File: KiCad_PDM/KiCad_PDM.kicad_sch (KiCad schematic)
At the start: 67 parts, among them J1 Conn_02x16_Top_Bottom, J2 6437288-1, J3 T66145145-1500, U1 74HC27D, U2 74HC27D, U3 74HC27D, U4 74HC27D, U5 KF33BDT-TR

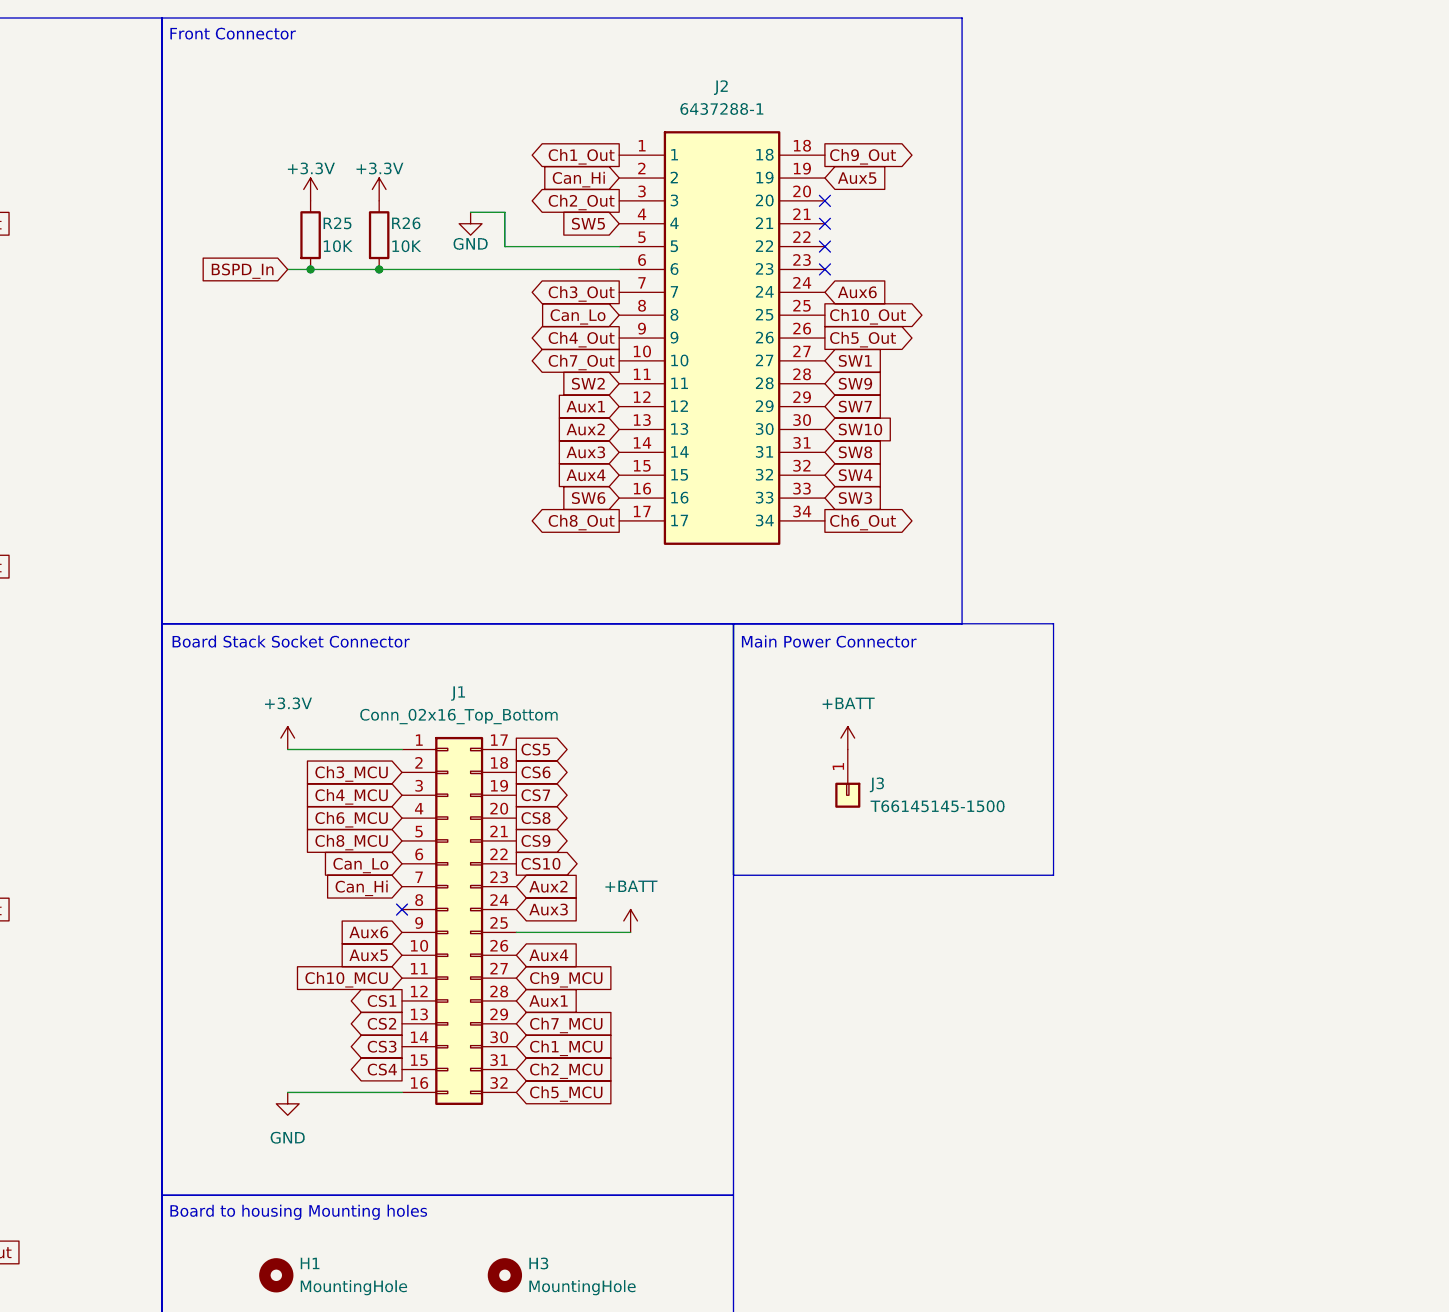
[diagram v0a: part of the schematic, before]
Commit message: MK1
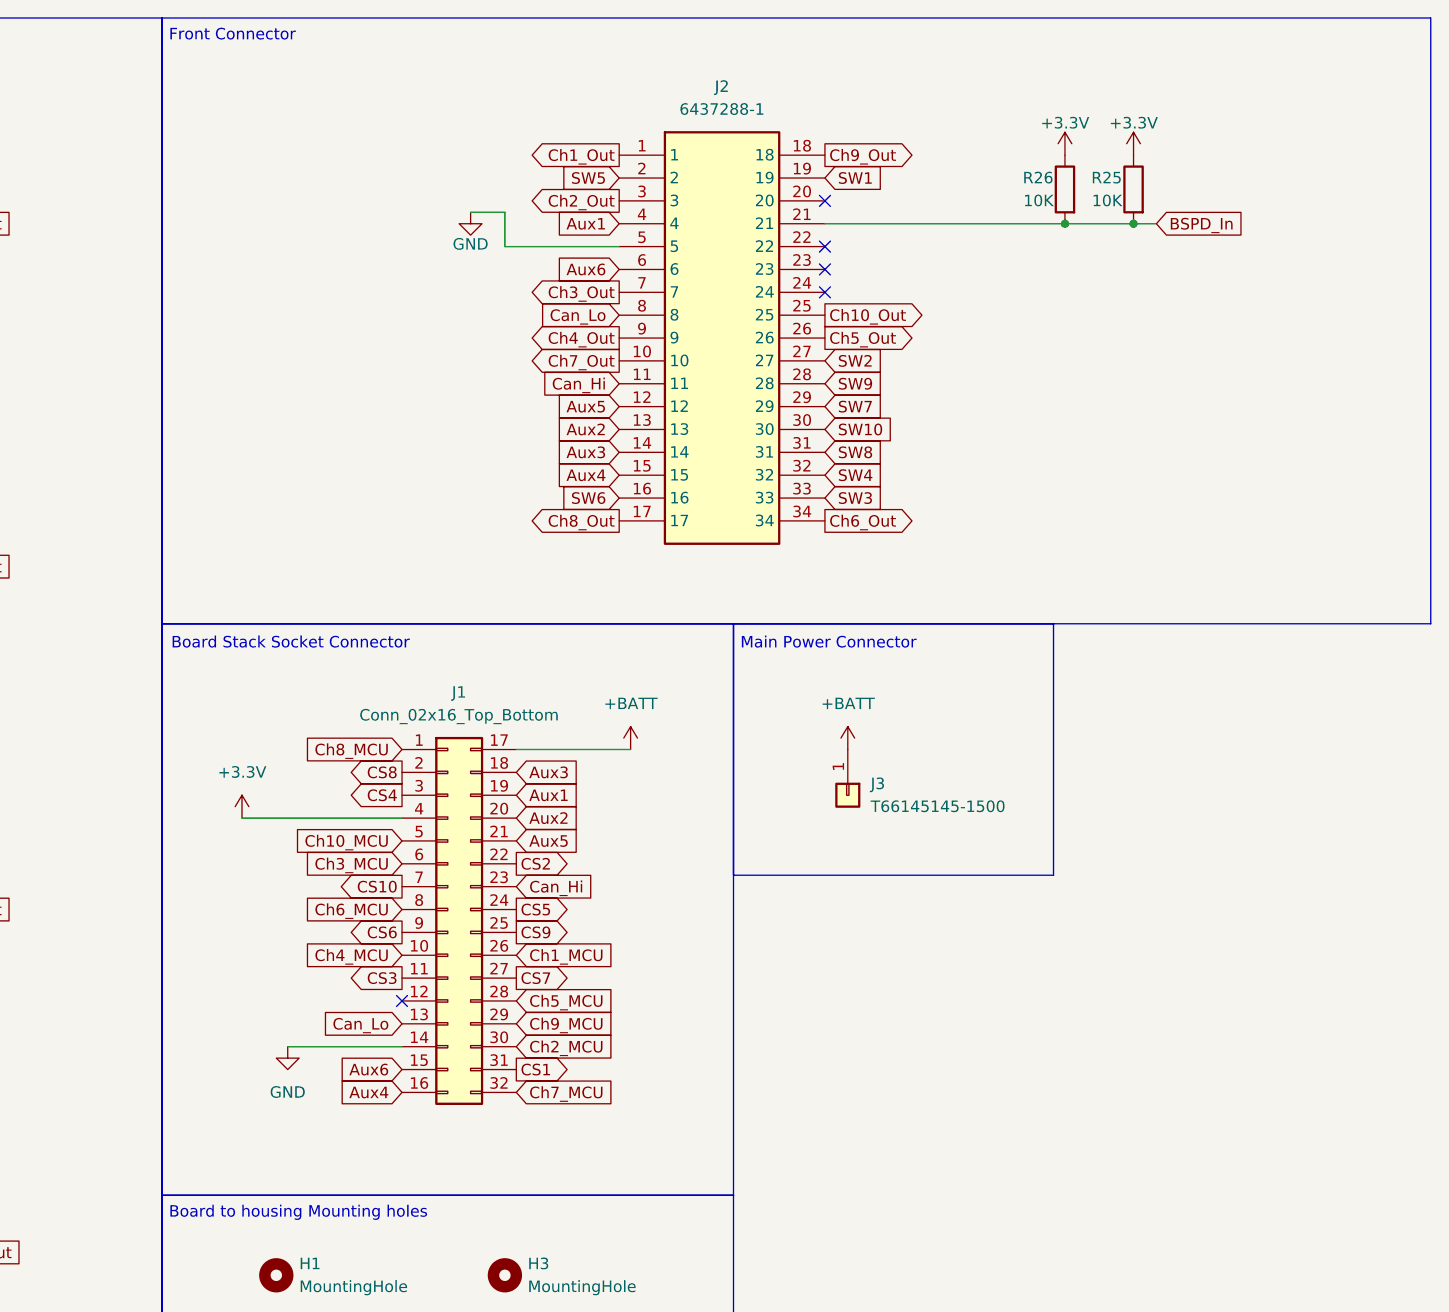
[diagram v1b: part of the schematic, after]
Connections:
- net +3.3V: now also J1.4 (Pin_4); no longer J1.1 (Pin_1)
- net +BATT: now also J1.17 (Pin_17); no longer J1.25 (Pin_25)
- net Aux1: now also J1.19 (Pin_19), J2.4; no longer J1.28 (Pin_28), J2.12
- net Aux2: now also J1.20 (Pin_20); no longer J1.23 (Pin_23)
- net Aux3: now also J1.18 (Pin_18); no longer J1.24 (Pin_24)
- net Aux4: now also J1.16 (Pin_16); no longer J1.26 (Pin_26)
- net Aux5: now also J1.21 (Pin_21), J2.12; no longer J1.10 (Pin_10), J2.19
- net Aux6: now also J1.15 (Pin_15), J2.6; no longer J1.9 (Pin_9), J2.24
- net BSPD_In: now also J2.21; no longer J2.6
- net CS1: now also J1.31 (Pin_31); no longer J1.12 (Pin_12)
- net CS10: now also J1.7 (Pin_7); no longer J1.22 (Pin_22)
- net CS2: now also J1.22 (Pin_22); no longer J1.13 (Pin_13)
- net CS3: now also J1.11 (Pin_11); no longer J1.14 (Pin_14)
- net CS4: now also J1.3 (Pin_3); no longer J1.15 (Pin_15)
- net CS5: now also J1.24 (Pin_24); no longer J1.17 (Pin_17)
- net CS6: now also J1.9 (Pin_9); no longer J1.18 (Pin_18)
- net CS7: now also J1.27 (Pin_27); no longer J1.19 (Pin_19)
- net CS8: now also J1.2 (Pin_2); no longer J1.20 (Pin_20)
- net CS9: now also J1.25 (Pin_25); no longer J1.21 (Pin_21)
- net Can_Hi: now also J1.23 (Pin_23), J2.11; no longer J1.7 (Pin_7), J2.2
- net Can_Lo: now also J1.13 (Pin_13); no longer J1.6 (Pin_6)
- net Ch10_MCU: now also J1.5 (Pin_5); no longer J1.11 (Pin_11)
- net Ch1_MCU: now also J1.26 (Pin_26); no longer J1.30 (Pin_30)
- net Ch2_MCU: now also J1.30 (Pin_30); no longer J1.31 (Pin_31)
- net Ch3_MCU: now also J1.6 (Pin_6); no longer J1.2 (Pin_2)
- net Ch4_MCU: now also J1.10 (Pin_10); no longer J1.3 (Pin_3)
- net Ch5_MCU: now also J1.28 (Pin_28); no longer J1.32 (Pin_32)
- net Ch6_MCU: now also J1.8 (Pin_8); no longer J1.4 (Pin_4)
- net Ch7_MCU: now also J1.32 (Pin_32); no longer J1.29 (Pin_29)
- net Ch8_MCU: now also J1.1 (Pin_1); no longer J1.5 (Pin_5)
- net Ch9_MCU: now also J1.29 (Pin_29); no longer J1.27 (Pin_27)
- net GND: now also J1.14 (Pin_14); no longer J1.16 (Pin_16)
- net SW1: now also J2.19; no longer J2.27
- net SW2: now also J2.27; no longer J2.11
- net SW5: now also J2.2; no longer J2.4
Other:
- moved on the sheet: R25, R26
